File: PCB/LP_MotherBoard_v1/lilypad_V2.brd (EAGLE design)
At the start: 63.5 x 53.3 mm, 28 parts, among them U2 INA169, X4 BQ24074

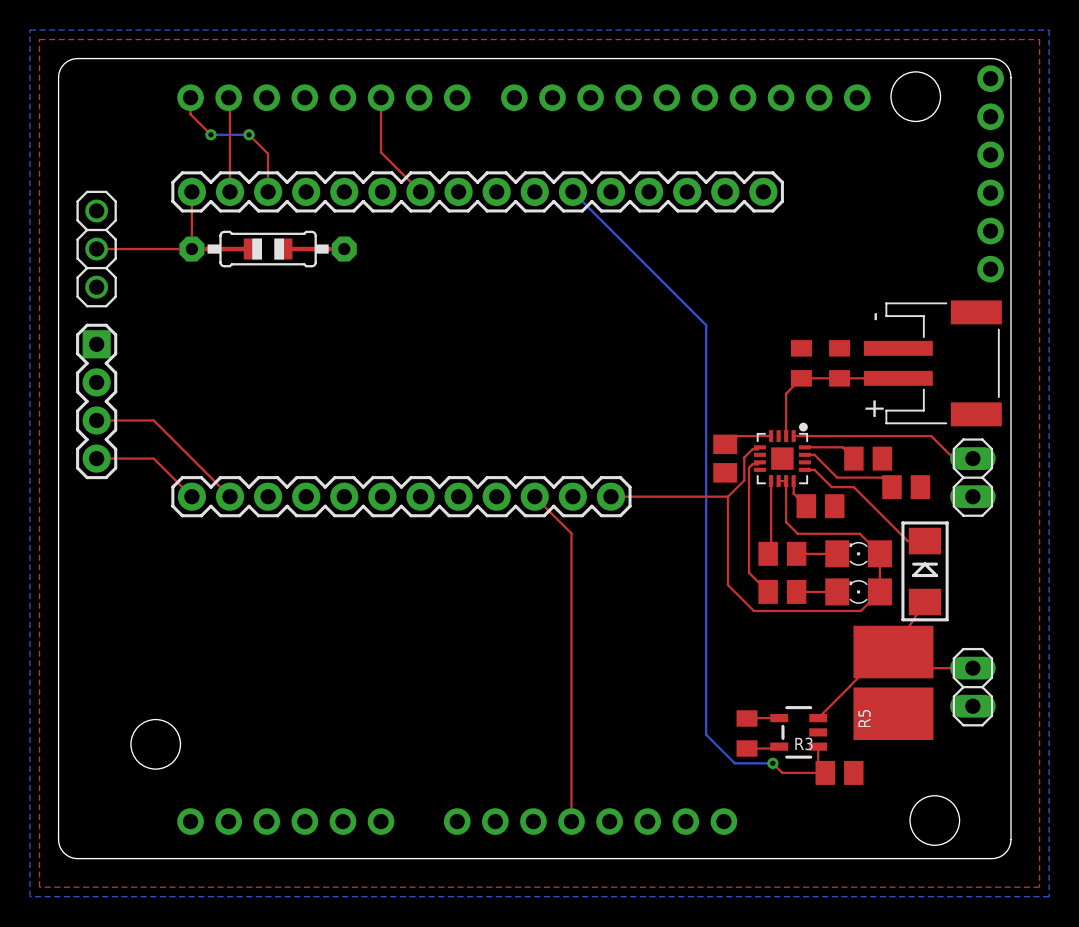
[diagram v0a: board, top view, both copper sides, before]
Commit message: Lilypad PCB Post Review and README
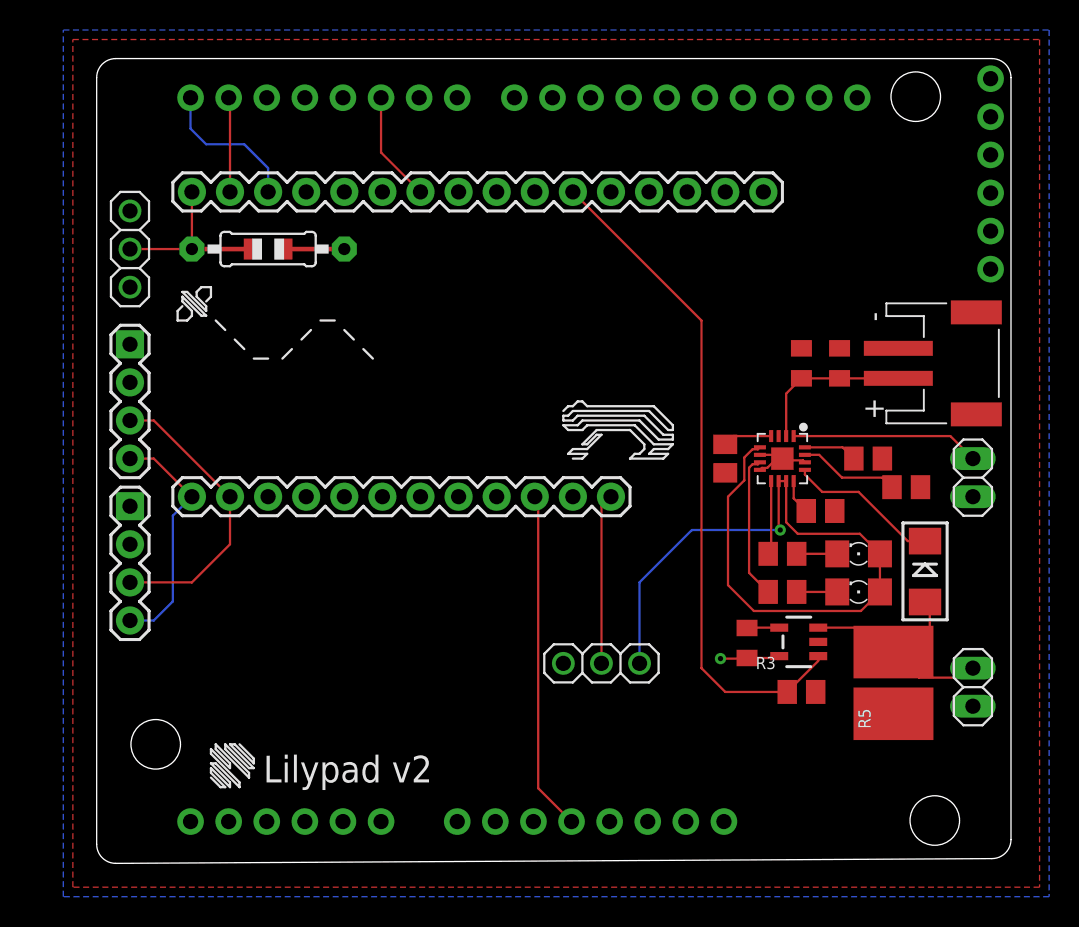
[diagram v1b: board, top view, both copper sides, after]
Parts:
- added J2: (no value), SparkFun-Connectors:1X04
- added JP1: (no value), adafruit:1X03
- moved C1 6.03 mm to (45.9, 14.4)
- moved U2 6.03 mm to (49.3, 14.4)
- moved R3 5.97 mm to (49.5, 11.1)
- moved J1 2.22 mm to (4.76, 34.3)
- moved JP7 2.22 mm to (4.76, 40.6)
- moved R1 0.32 mm to (50.8, 23.2)
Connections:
- new net VIN: HP2.1, JP1.2
- net GND: now also J2.2
- net SCL: now also J2.3
- net SDA: now also J2.4
- net VBAT: now also JP1.3; no longer HP2.1
- net VCC: now also J2.1
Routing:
- net VBAT: track 42.6 -> 54.3 mm, vias 0 -> 1
- net VIN: track 0.00 -> 11.4 mm
- net SDA: track 7.40 -> 16.1 mm
- net SCL: track 11.0 -> 19.7 mm
- net A1: track 50.8 -> 44.9 mm, vias 1 -> 0
- net GND: track 2.16 -> 7.17 mm
- net CHARGER_IN: track 16.9 -> 21.0 mm
- net TMP_PRB: track 9.94 -> 7.71 mm
- net VCC: track 2.20 -> 3.98 mm, vias 0 -> 1
- net RX: vias 2 -> 0
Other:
- board size 63.5 x 53.3 mm -> 61 x 53.7 mm
- board text added: "Lilypad v2"
